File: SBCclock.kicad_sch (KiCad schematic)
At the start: 19 parts, among them J1 Conn_01x06_Male, J2 Conn_01x06_Male, U1 74HC14, U2 74HCT163, U3 74HCT74, Y1 25.175MHz

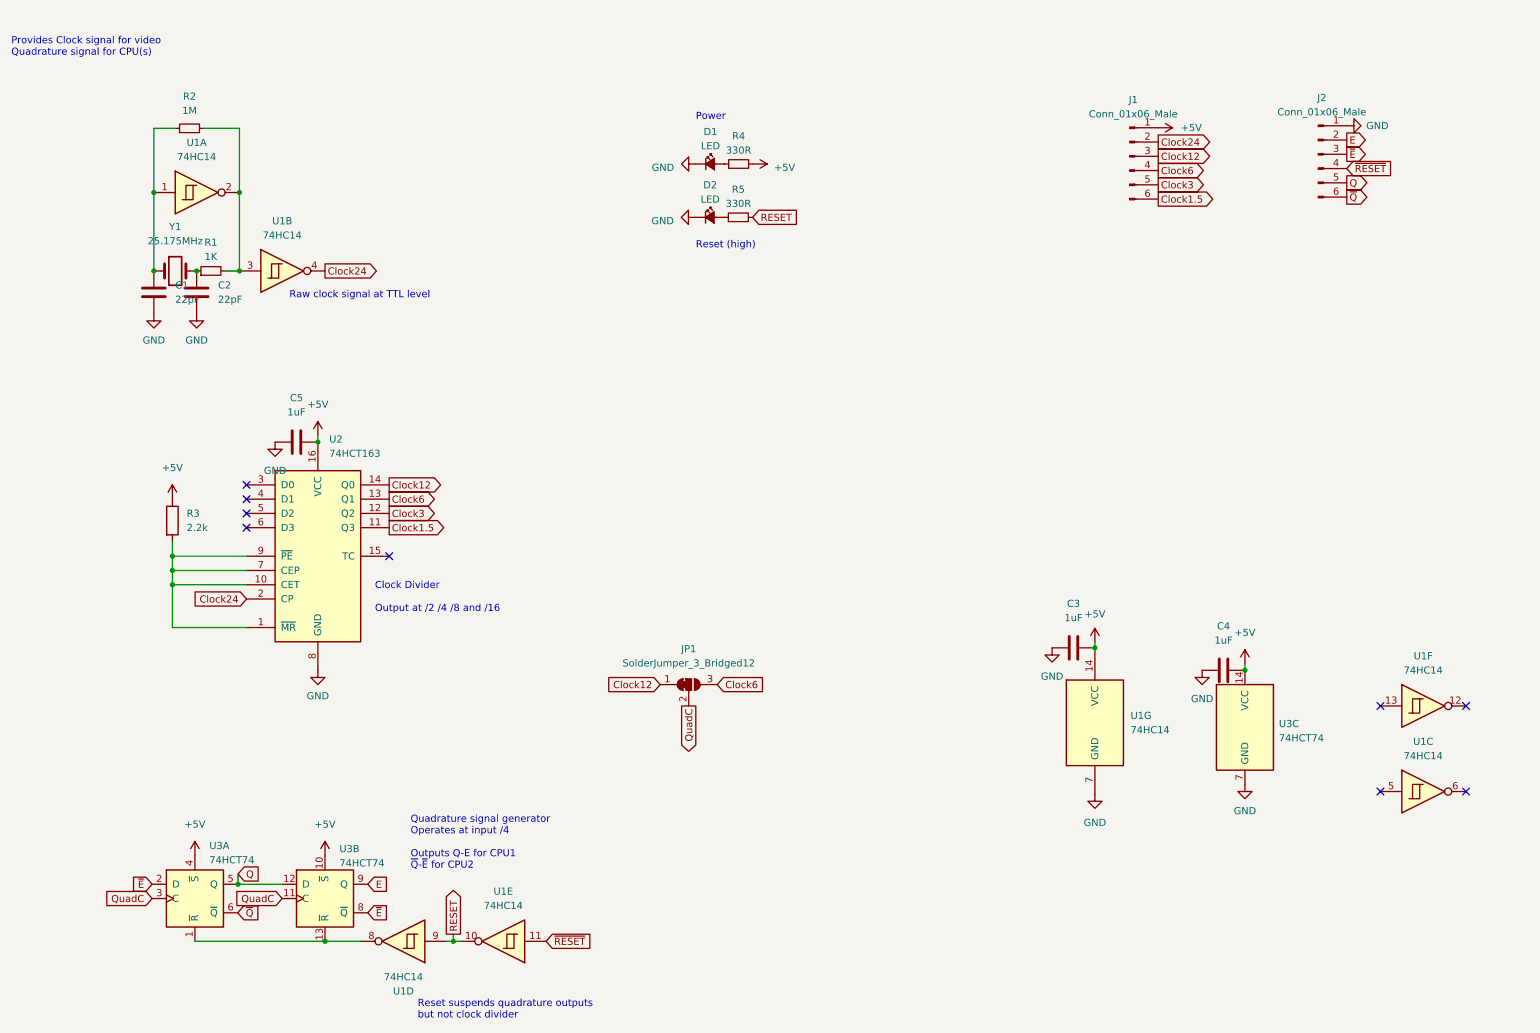
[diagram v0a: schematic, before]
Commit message: v2 board
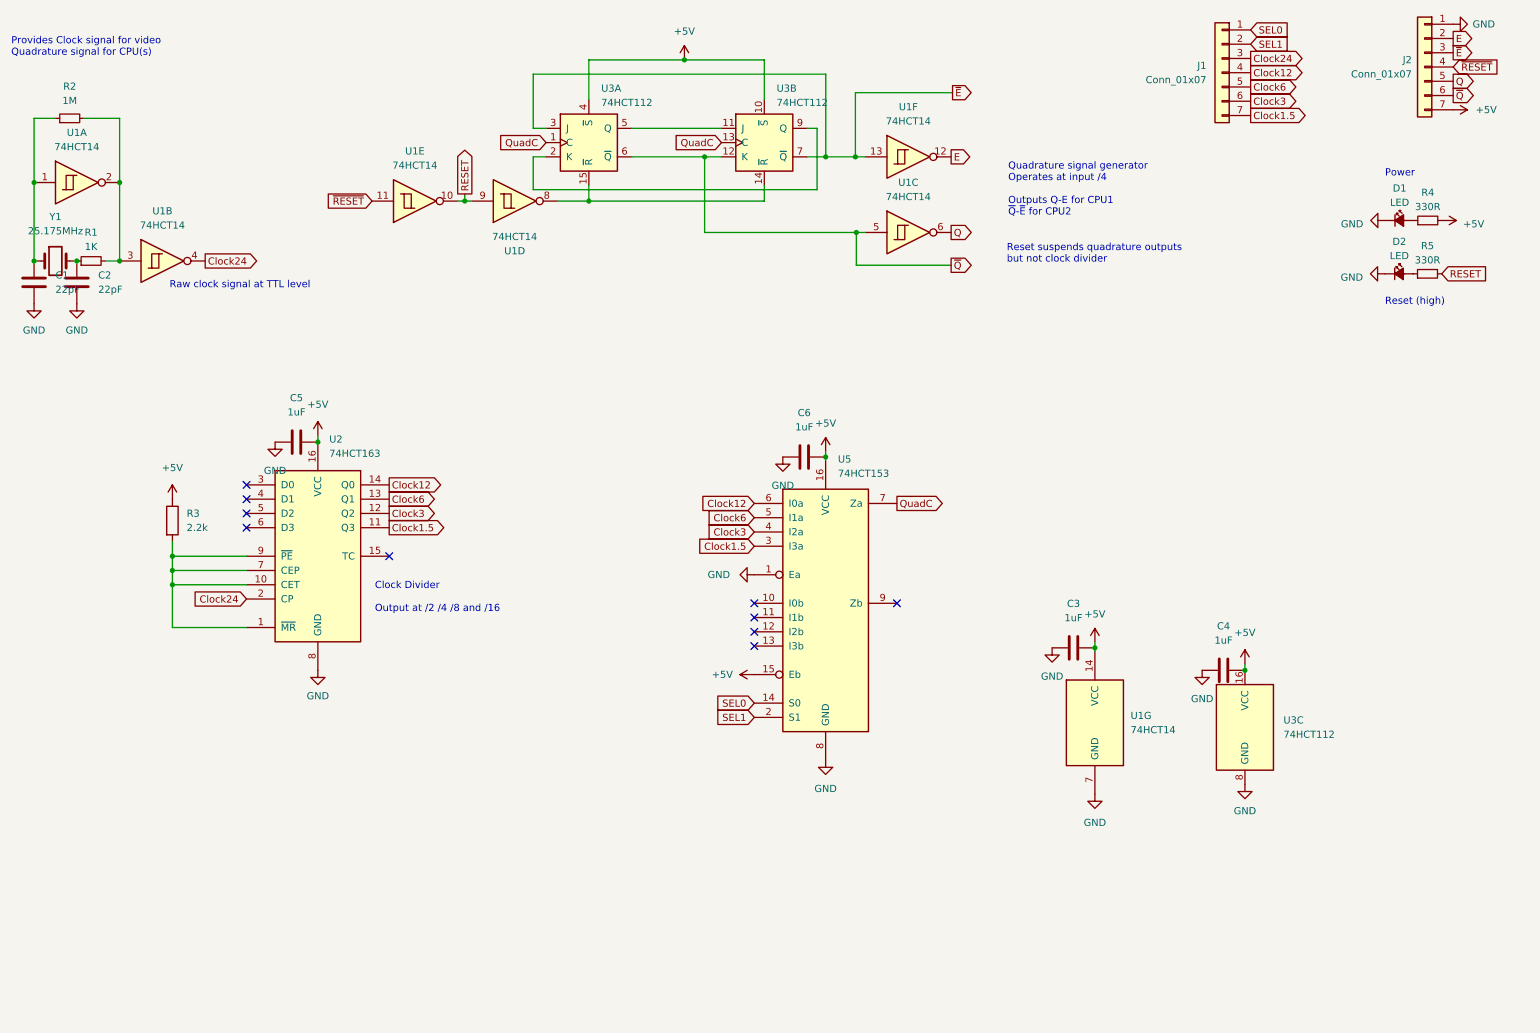
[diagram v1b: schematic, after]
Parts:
- removed J1, J2: Conn_01x06_Male, Connector_PinHeader_2.54mm:PinHeader_1x06_P2.54mm_Vertical, symbol Connector:Conn_01x06_Male
- removed JP1: SolderJumper_3_Bridged12, Jumper:SolderJumper-3_P1.3mm_Bridged12_Pad1.0x1.5mm, symbol Jumper:SolderJumper_3_Bridged12
- removed U3: 74HCT74, Package_SO:SOIC-14_3.9x8.7mm_P1.27mm, symbol 74xx:74HC74
- added C6: 1uF, Capacitor_SMD:C_0805_2012Metric_Pad1.18x1.45mm_HandSolder, symbol Device:C
- added J1, J2: Conn_01x07, Connector_PinHeader_2.54mm:PinHeader_1x07_P2.54mm_Vertical, symbol Connector_Generic:Conn_01x07
- added U3: 74HCT112, Package_SO:SOIC-16_3.9x9.9mm_P1.27mm, symbol 74xx:74LS112
- added U5: 74HCT153, Package_SO:SOIC-16_3.9x9.9mm_P1.27mm, symbol 74xx:74LS153
- U1: value 74HC14 -> 74HCT14; DigiKey (none) -> 296-14864-1-ND
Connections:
- net +5V: now also C6.1, J2.7 (Pin_7), U3.10 (~{S}), U3.16 (VCC), U3.4 (~{S}), U5.15 (Eb), U5.16 (VCC)
- net Clock1.5: now also J1.7 (Pin_7), U5.3 (I3a)
- net Clock12: now also J1.4 (Pin_4), U5.6 (I0a)
- net Clock24: now also J1.3 (Pin_3)
- net Clock3: now also J1.6 (Pin_6), U5.4 (I2a)
- net Clock6: now also J1.5 (Pin_5), U5.5 (I1a)
- net E: now also U1.12, J2.2 (Pin_2)
- net GND: now also C6.2, J2.1 (Pin_1), U3.8 (GND), U5.1 (Ea), U5.8 (GND)
- net Q: now also U1.6, J2.5 (Pin_5)
- net QuadC: now also U3.1 (C), U3.13 (C), U5.7 (Za)
- net ~{E}: now also U1.13, J2.3 (Pin_3), U3.3 (J), U3.7 (~{Q})
- net ~{Q}: now also U1.5, J2.6 (Pin_6), U3.12 (K), U3.6 (~{Q})
- net ~{RESET}: now also J2.4 (Pin_4)
- net at U1.8: now also U3.14 (~{R}), U3.15 (~{R})
- new net: U3.2 (K), U3.9 (Q)
- new net: U3.11 (J), U3.5 (Q)
- new net SEL0: J1.1 (Pin_1), U5.14 (S0)
- new net SEL1: J1.2 (Pin_2), U5.2 (S1)
- no-connect marks 9 -> 10
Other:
- moved on the sheet: C1, C2, D1, D2, R1, R2, R4, R5, U1A, U1B, U1C, U1D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
